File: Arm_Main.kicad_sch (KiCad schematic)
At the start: 33 parts, among them IC1 TLP559_F_, J1 Conn_01x03_Socket, J2 Conn_01x02_Pin, J4 Conn_01x03_Pin, J5 Conn_01x03_Pin, J6 Conn_01x03_Pin, SW2 SW_SPDT, U1 RASPBERRY_PI_ZERO_2_W, U2 TLP2531, U3 TLP2531

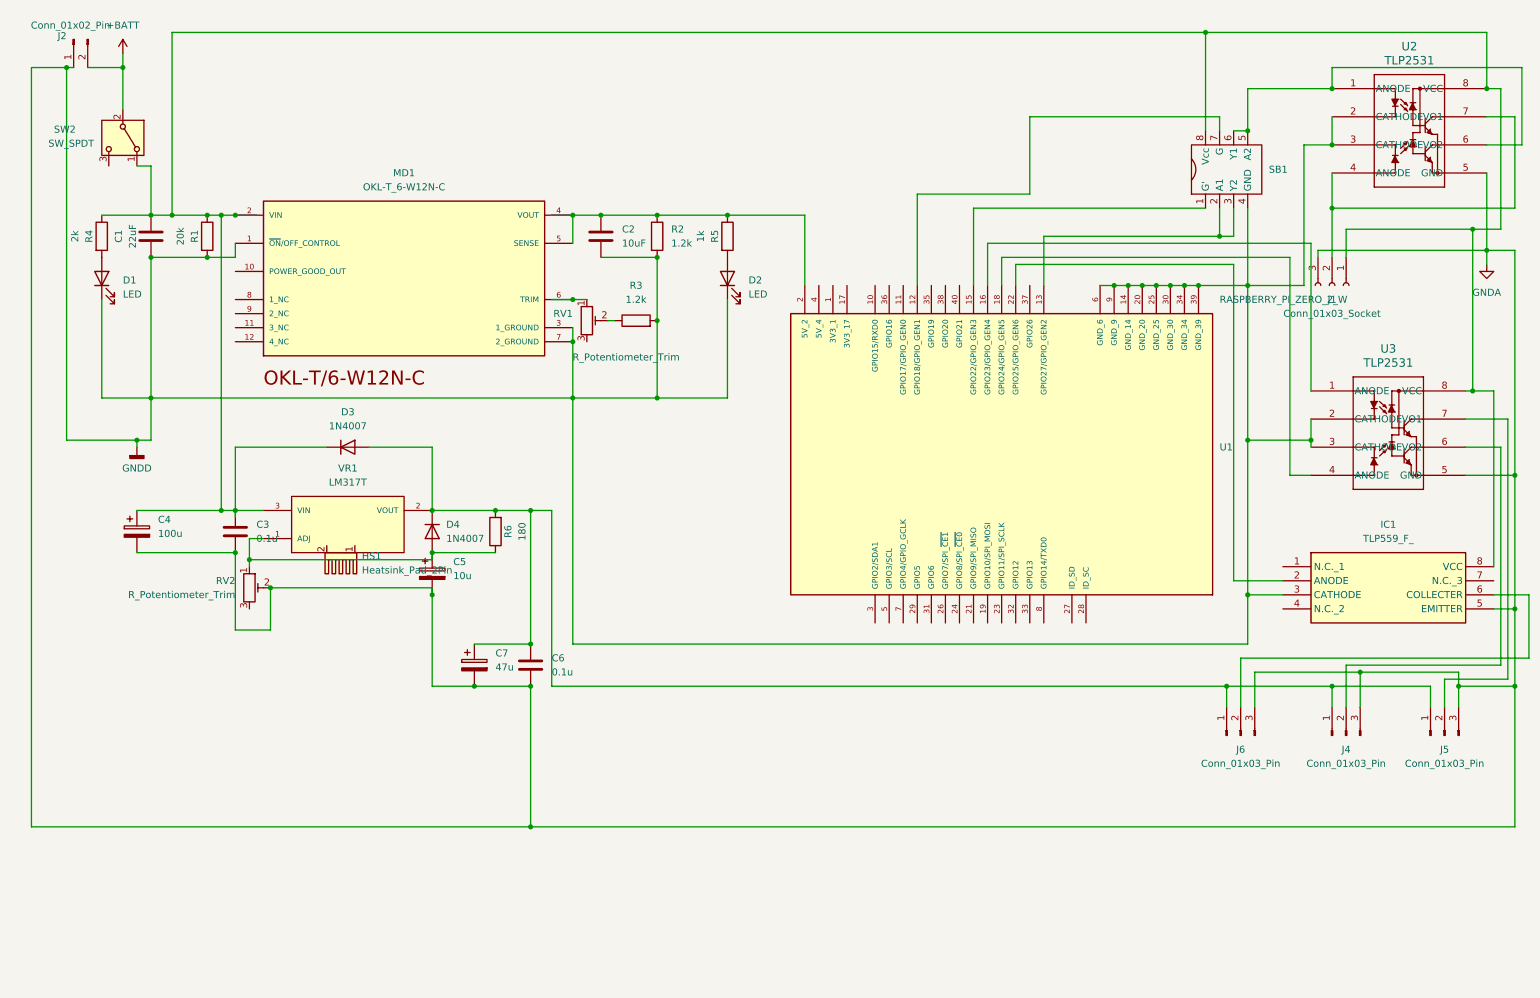
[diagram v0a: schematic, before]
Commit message: ver6
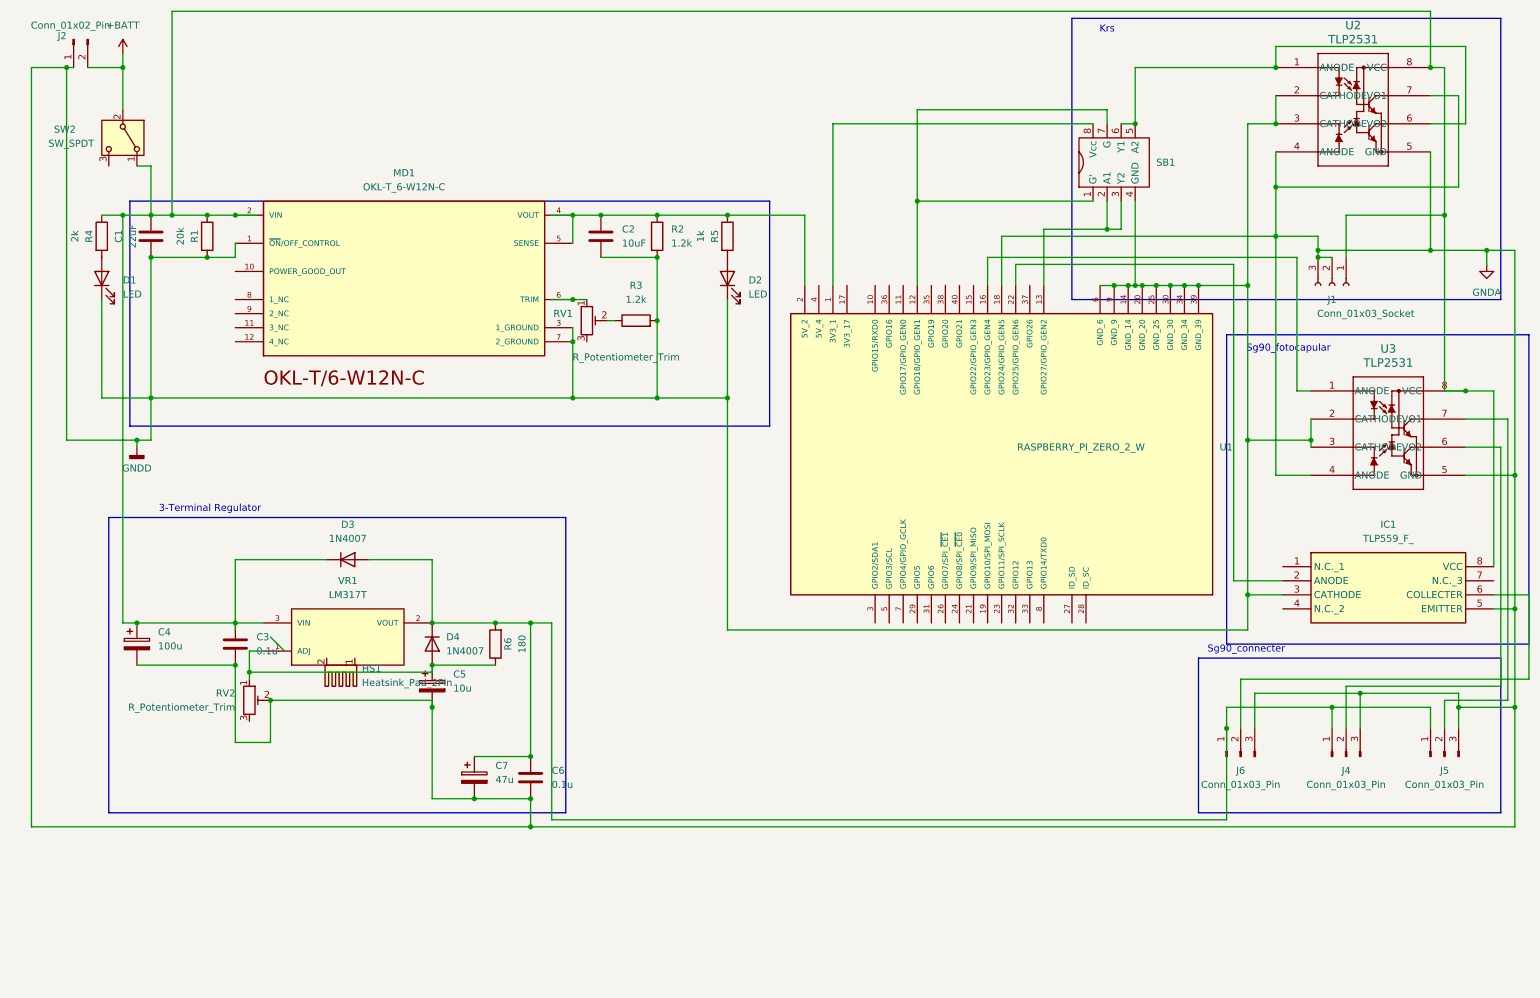
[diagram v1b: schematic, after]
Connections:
- net GNDA: now also J1.2 (Pin_2), U1.18 (GPIO24/GPIO_GEN5), U2.4 (ANODE), U2.7 (VO1), U3.4 (ANODE)
- net at C1.1, C3.1, C4.1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: no longer SB1.8 (Vcc)
- net at U1.1 (3V3_1): now also SB1.8 (Vcc)
- net at SB1.7 (G), U1.12 (GPIO18/GPIO_GEN1): now also SB1.1 (G')
- net at U1.15 (GPIO22/GPIO_GEN3): no longer SB1.1 (G')
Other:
- note added: "3-Terminal Regulator"
- note added: "Krs"
- note added: "Sg90_connecter"
- note added: "Sg90_fotocapular"
- moved on the sheet: C3, C4, C5, C6, C7, D3, D4, HS1, J4, J5, J6, R6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

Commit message: Ver_7
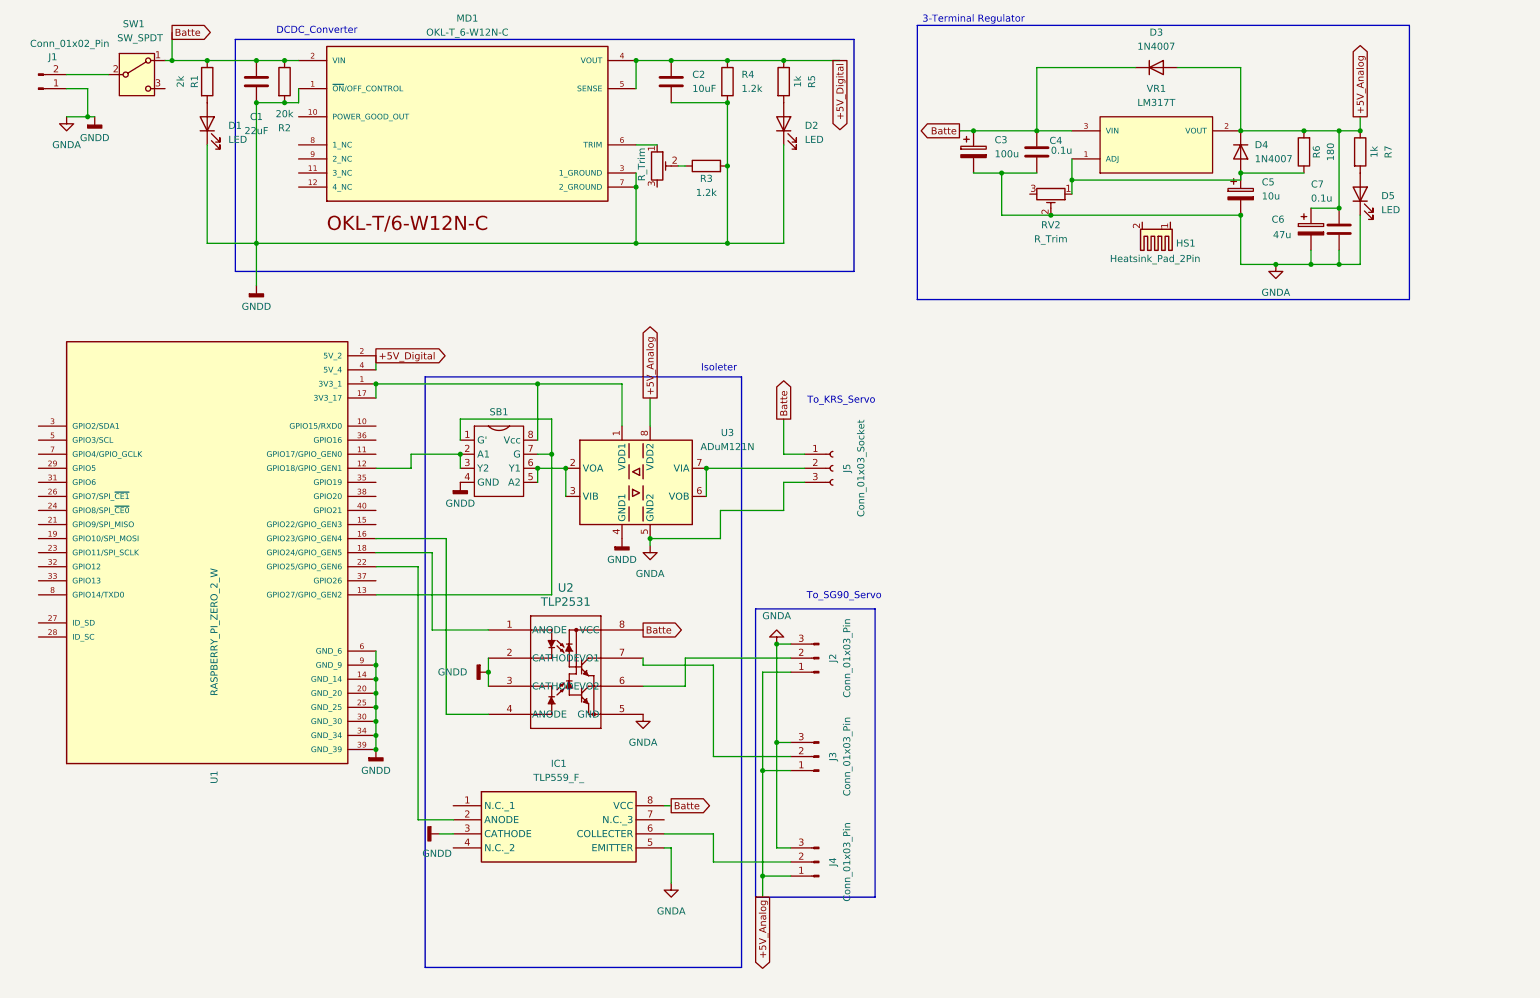
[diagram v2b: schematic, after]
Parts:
- removed C3, C6: 0.1u, Capacitor_THT:C_Disc_D5.1mm_W3.2mm_P5.00mm, symbol Device:C
- removed C4: 100u, Capacitor_THT:CP_Radial_D5.0mm_P2.50mm, symbol Device:C_Polarized
- removed C7: 47u, Capacitor_THT:CP_Radial_D5.0mm_P2.50mm, symbol Device:C_Polarized
- removed J1: Conn_01x03_Socket, Connector_JST:JST_XH_B3B-XH-A_1x03_P2.50mm_Vertical, symbol Connector:Conn_01x03_Socket
- removed J2: Conn_01x02_Pin, Connector_AMASS:AMASS_XT30U-F_1x02_P5.0mm_Vertical, symbol Connector:Conn_01x02_Pin
- removed J5, J6: Conn_01x03_Pin, Connector_PinHeader_2.54mm:PinHeader_1x03_P2.54mm_Vertical, symbol Connector:Conn_01x03_Pin
- removed SW2: SW_SPDT, Togle_original:TogleSW3pin, symbol Switch:SW_SPDT
- removed U3: TLP2531, U_DIP8_11-10C4S_TOS, symbol TLP2531_sym:TLP2531
- added C3: 100u, Capacitor_THT:CP_Radial_D5.0mm_P2.50mm, symbol Device:C_Polarized
- added C4, C7: 0.1u, Capacitor_THT:C_Disc_D5.1mm_W3.2mm_P5.00mm, symbol Device:C
- added C6: 47u, Capacitor_THT:CP_Radial_D5.0mm_P2.50mm, symbol Device:C_Polarized
- added D5: LED, LED_THT:LED_D3.0mm, symbol Device:LED
- added J1: Conn_01x02_Pin, Connector_AMASS:AMASS_XT30U-F_1x02_P5.0mm_Vertical, symbol Connector:Conn_01x02_Pin
- added J2, J3: Conn_01x03_Pin, Connector_PinHeader_2.54mm:PinHeader_1x03_P2.54mm_Vertical, symbol Connector:Conn_01x03_Pin
- added J5: Conn_01x03_Socket, Connector_JST:JST_XH_B3B-XH-A_1x03_P2.50mm_Vertical, symbol Connector:Conn_01x03_Socket
- added R7: 1k, Resistor_THT:R_Axial_DIN0207_L6.3mm_D2.5mm_P10.16mm_Horizontal, symbol Device:R
- added SW1: SW_SPDT, Togle_original:TogleSW3pin, symbol Switch:SW_SPDT
- added U3: ADuM121N, Package_SO:SOIC-8_3.9x4.9mm_P1.27mm, symbol Isolator:ADuM121N
- R1: value 20k -> 2k
- R2: value 1.2k -> 20k
- R4: value 2k -> 1.2k
- RV1, RV2: value R_Potentiometer_Trim -> R_Trim
- U2: footprint ul_TLP2531:U_DIP8_11-10C4S_TOS -> U_DIP8_11-10C4S_TOS
- VR1: footprint NJM317:TO254P1054X470X1955-3 -> Njm317_original:TO254P1054X470X1955-3
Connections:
- net GNDA: now also R4.2, C3.2, C4.2, C6.2, C7.2, D5.1 (K), J1.1 (Pin_1), J2.3 (Pin_3), J3.3 (Pin_3), J5.3 (Pin_3), U3.4 (GND1), U3.5 (GND2); no longer R1.2, U1.18 (GPIO24/GPIO_GEN5), U2.4 (ANODE), U2.7 (VO1)
- net Batte: now reaches C1.1, D3.1 (K), IC1.8 (VCC), MD1.2 (VIN), R1.1, U2.8 (VCC), VR1.3 (VIN)
- net Batte: now also R2.1, C3.1, C4.1, J5.1 (Pin_1), SW1.1 (A); no longer R4.1
- net at D1.2 (A): now also R1.2; no longer R4.2
- net +5V_Digital: now reaches C2.1, MD1.4 (VOUT), MD1.5 (SENSE), R5.1, U1.2 (5V_2)
- net +5V_Digital: now also R4.1, U1.4 (5V_4); no longer R2.1
- net at U1.16 (GPIO23/GPIO_GEN4): now also U2.4 (ANODE)
- net at J4.2 (Pin_2): now also IC1.6 (COLLECTER)
- net at SB1.8 (Vcc), U1.1 (3V3_1): now also U1.17 (3V3_17), U3.1 (VDD1)
- net at SB1.1 (G'), SB1.7 (G): now also U1.13 (GPIO27/GPIO_GEN2); no longer U1.12 (GPIO18/GPIO_GEN1)
- net at SB1.2 (A1), SB1.3 (Y2): now also U1.12 (GPIO18/GPIO_GEN1); no longer U1.13 (GPIO27/GPIO_GEN2)
- net +5V_Analog: now reaches D3.2 (A), D4.1 (K), J4.1 (Pin_1), R6.2, VR1.2 (VOUT)
- net +5V_Analog: now also C6.1, C7.1, J2.1 (Pin_1), J3.1 (Pin_1), R7.1, U3.8 (VDD2)
- net at SB1.5 (A2), SB1.6 (Y1): now also U3.2 (VOA), U3.3 (VIB); no longer U2.1 (ANODE), U2.6 (VO2)
- new net: J2.2 (Pin_2), U2.6 (VO2)
- new net: J3.2 (Pin_2), U2.7 (VO1)
- new net: J1.2 (Pin_2), SW1.2 (B)
- new net: U1.18 (GPIO24/GPIO_GEN5), U2.1 (ANODE)
- new net: J5.2 (Pin_2), U3.6 (VOB), U3.7 (VIA)
- new net: D5.2 (A), R7.2
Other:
- note added: "DCDC_Converter"
- note added: "Isoleter"
- note added: "To_KRS_Servo"
- note added: "To_SG90_Servo"
- note removed: "Krs"
- note removed: "Sg90_connecter"
- note removed: "Sg90_fotocapular"
